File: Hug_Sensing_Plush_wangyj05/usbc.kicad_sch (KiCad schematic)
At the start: 5 parts, among them J1 USB_C_Receptacle_USB2.0_16P, U5 USBLC6-2SC6

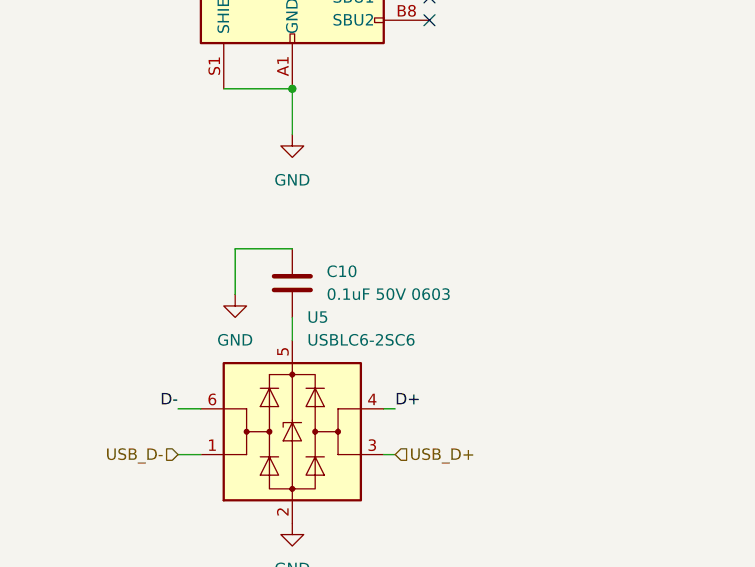
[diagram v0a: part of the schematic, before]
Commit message: Hug-Sensing IoT Plush
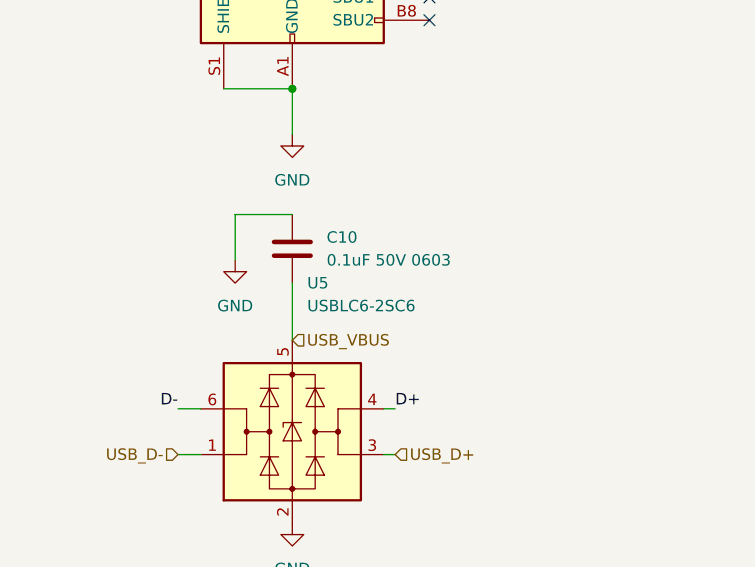
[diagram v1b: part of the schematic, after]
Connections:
- net USB_VBUS: now also C10.2, U5.5 (VBUS)
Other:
- moved on the sheet: C10
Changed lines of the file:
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@@
     (stroke (width 0) (type default))
   )
-  (wire (pts (xy 50.8 138.43) (xy 50.8 133.35))
+  (wire (pts (xy 50.8 134.62) (xy 50.8 129.54))
     (stroke (width 0) (type default))
   )
@@
     (stroke (width 0) (type default))
   )
-  (wire (pts (xy 50.8 133.35) (xy 57.15 133.35))
-    (stroke (width 0) (type default))
-  )
-  (wire (pts (xy 57.15 140.97) (xy 57.15 143.51))
+  (wire (pts (xy 50.8 129.54) (xy 57.15 129.54))
     (stroke (width 0) (type default))
   )
   (wire (pts (xy 68.58 151.13) (xy 67.31 151.13))
+    (stroke (width 0) (type default))
+  )
+  (wire (pts (xy 57.15 137.16) (xy 57.15 143.51))
     (stroke (width 0) (type default))
   )
@@
     (effects (font (size 1.27 1.27)) (justify left))
   )
+  (hierarchical_label "USB_VBUS" (shape input) (at 57.15 143.51 0) (fields_autoplaced)
+    (effects (font (size 1.27 1.27)) (justify left))
+  )
   (symbol (lib_id "Power_Protection:USBLC6-2SC6") (at 57.15 153.67 0) (unit 1)
-    (in_bom yes) (on_board yes) (dnp no) (fields_autoplaced)
-    (property "Reference" "U5" (at 58.8011 140.97 0)
-      (effects (font (size 1.27 1.27)) (justify left))
-    )
-    (property "Value" "USBLC6-2SC6" (at 58.8011 143.51 0)
+    (in_bom yes) (on_board yes) (dnp no)
+    (property "Reference" "U5" (at 58.8011 137.16 0)
+      (effects (font (size 1.27 1.27)) (justify left))
+    )
+    (property "Value" "USBLC6-2SC6" (at 58.8011 139.7 0)
       (effects (font (size 1.27 1.27)) (justify left))
     )
@@
     )
   )
-  (symbol (lib_id "power:GND") (at 50.8 138.43 0) (unit 1)
-    (in_bom yes) (on_board yes) (dnp no) (fields_autoplaced)
-    (property "Reference" "#PWR027" (at 50.8 144.78 0)
-      (effects (font (size 1.27 1.27)) hide)
-    )
-    (property "Value" "GND" (at 50.8 143.51 0)
-      (effects (font (size 1.27 1.27)))
-    )
-    (property "Footprint" "" (at 50.8 138.43 0)
-      (effects (font (size 1.27 1.27)) hide)
-    )
-    (property "Datasheet" "" (at 50.8 138.43 0)
+  (symbol (lib_id "power:GND") (at 50.8 134.62 0) (unit 1)
+    (in_bom yes) (on_board yes) (dnp no) (fields_autoplaced)
+    (property "Reference" "#PWR027" (at 50.8 140.97 0)
+      (effects (font (size 1.27 1.27)) hide)
+    )
+    (property "Value" "GND" (at 50.8 139.7 0)
+      (effects (font (size 1.27 1.27)))
+    )
+    (property "Footprint" "" (at 50.8 134.62 0)
+      (effects (font (size 1.27 1.27)) hide)
+    )
+    (property "Datasheet" "" (at 50.8 134.62 0)
       (effects (font (size 1.27 1.27)) hide)
     )
@@
     )
   )
-  (symbol (lib_id "Device:C") (at 57.15 137.16 0) (unit 1)
-    (in_bom yes) (on_board yes) (dnp no) (fields_autoplaced)
-    (property "Reference" "C10" (at 60.96 135.89 0)
-      (effects (font (size 1.27 1.27)) (justify left))
-    )
-    (property "Value" "0.1uF 50V 0603" (at 60.96 138.43 0)
-      (effects (font (size 1.27 1.27)) (justify left))
-    )
-    (property "Footprint" "Capacitor_SMD:C_0603_1608Metric_Pad1.08x0.95mm_HandSolder" (at 58.1152 140.97 0)
-      (effects (font (size 1.27 1.27)) hide)
-    )
-    (property "Datasheet" "https://mm.digikey.com/Volume0/opasdata/d220001/medias/docus/658/CL10B104KB8NNNL_Spec.pdf" (at 57.15 137.16 0)
-      (effects (font (size 1.27 1.27)) hide)
-    )
-    (property "Digikey PN" "1276-CL10B104KB8NNNLCT-ND" (at 57.15 137.16 0)
-      (effects (font (size 1.27 1.27)) hide)
-    )
-    (property "MPN" "CL10B104KB8NNNL" (at 57.15 137.16 0)
-      (effects (font (size 1.27 1.27)) hide)
-    )
+  (symbol (lib_id "Device:C") (at 57.15 133.35 0) (unit 1)
+    (in_bom yes) (on_board yes) (dnp no) (fields_autoplaced)
+    (property "Reference" "C10" (at 60.96 132.08 0)
+      (effects (font (size 1.27 1.27)) (justify left))
+    )
+    (property "Value" "0.1uF 50V 0603" (at 60.96 134.62 0)
+      (effects (font (size 1.27 1.27)) (justify left))
+    )
+    (property "Footprint" "Capacitor_SMD:C_0603_1608Metric_Pad1.08x0.95mm_HandSolder" (at 58.1152 137.16 0)
+      (effects (font (size 1.27 1.27)) hide)
+    )
+    (property "Datasheet" "https://mm.digikey.com/Volume0/opasdata/d220001/medias/docus/658/CL10B104KB8NNNL_Spec.pdf" (at 57.15 133.35 0)
+      (effects (font (size 1.27 1.27)) hide)
+    )
+    (property "Digikey PN" "1276-CL10B104KB8NNNLCT-ND" (at 57.15 133.35 0)
+      (effects (font (size 1.27 1.27)) hide)
+    )
+    (property "MPN" "CL10B104KB8NNNL" (at 57.15 133.35 0)
+      (effects (font (size 1.27 1.27)) hide)
+    )
